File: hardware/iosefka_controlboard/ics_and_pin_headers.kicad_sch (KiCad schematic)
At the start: 18 parts, among them J1 Conn_01x10, J2 Conn_01x10, U2 MCP23017_SP, U3 MCP23017_SP, U4 4051, U5 4051

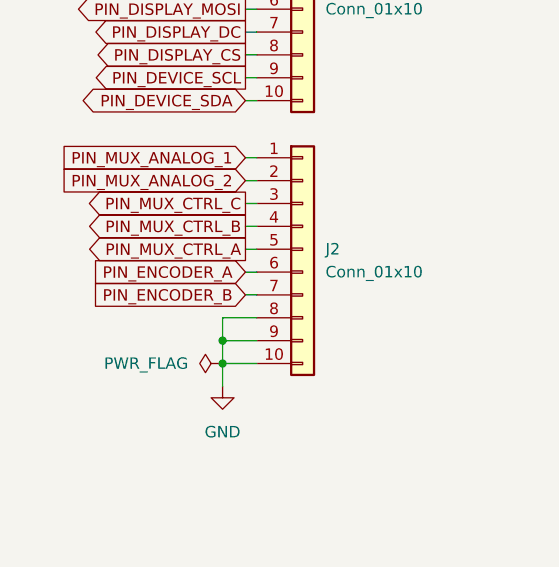
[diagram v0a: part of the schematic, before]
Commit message: added docs
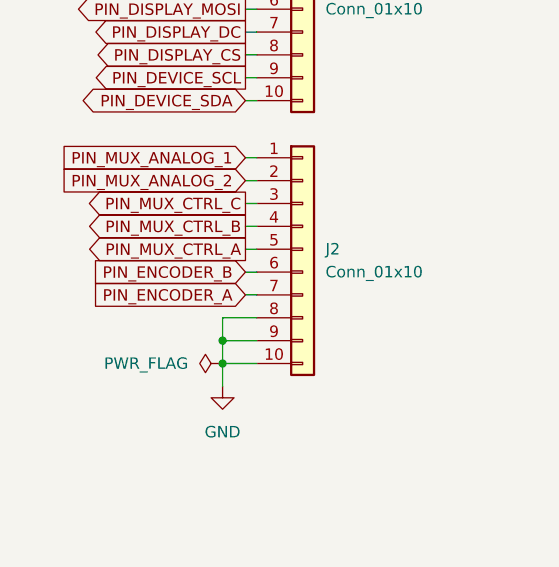
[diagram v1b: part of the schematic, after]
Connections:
- net PIN_ENCODER_A: now also J2.7 (Pin_7); no longer J2.6 (Pin_6)
- net PIN_ENCODER_B: now also J2.6 (Pin_6); no longer J2.7 (Pin_7)
